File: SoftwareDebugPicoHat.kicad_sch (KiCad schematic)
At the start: 13 parts, among them J1 35362-0950, J2 Conn_Coaxial, J3 USB_C_Receptacle_USB2.0_14P, J4 Conn_Coaxial, J5 Conn_01x04_Pin, U1 RFM98PW, U3 LORA1280F27-TCXO

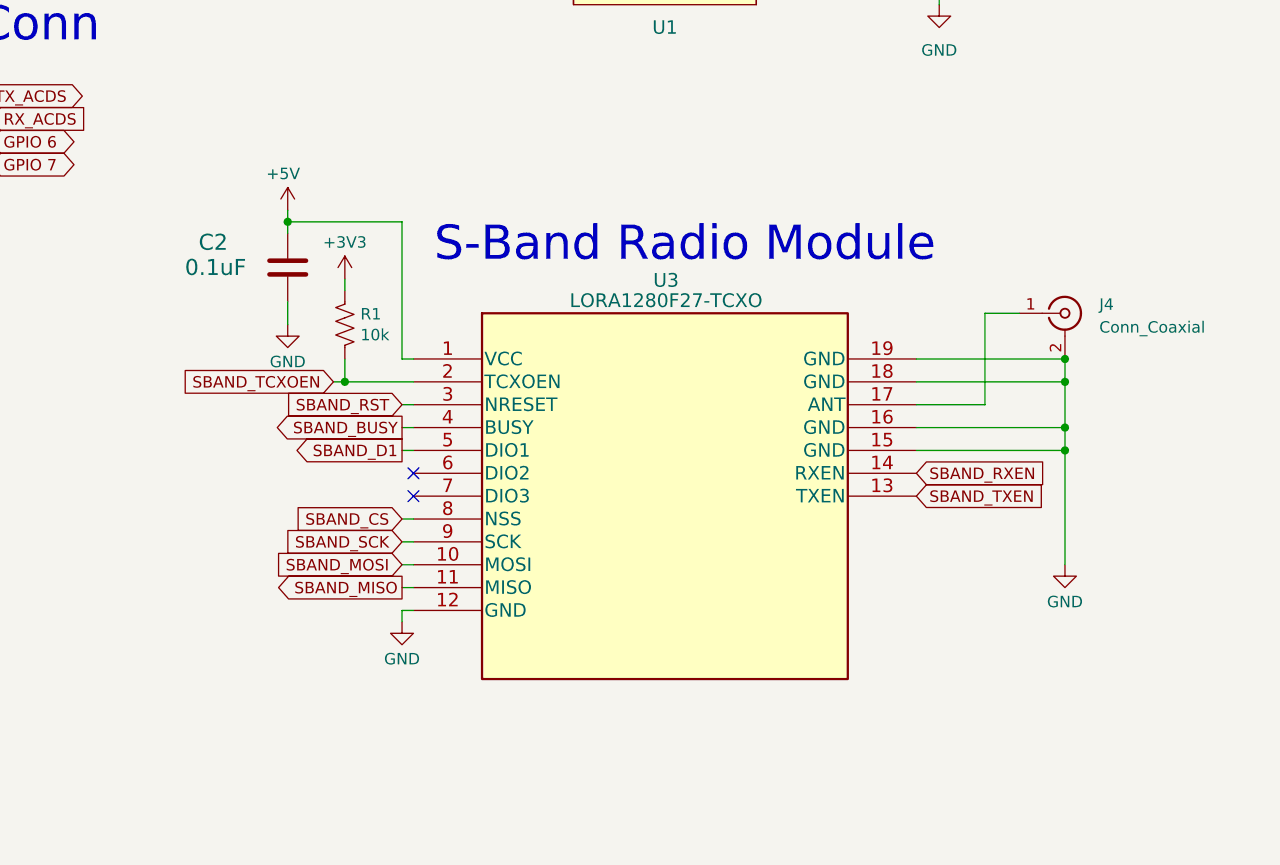
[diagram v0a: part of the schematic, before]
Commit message: Solving Samwise
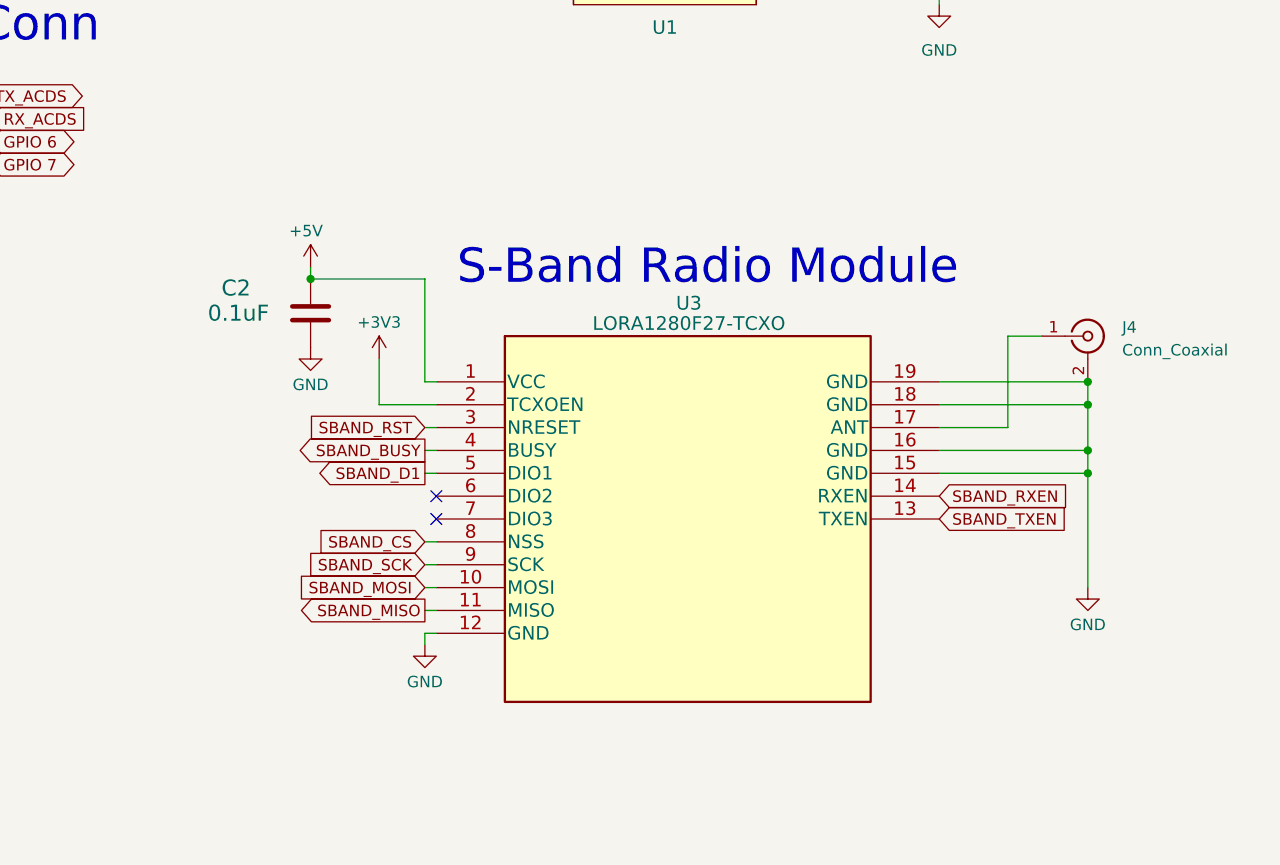
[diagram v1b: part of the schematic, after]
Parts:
- removed R1: 10k, Resistor_SMD:R_0603_1608Metric, symbol Device:R_US
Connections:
- net SBAND_TCXOEN is gone; now on net +3V3: U3.2 (TCXOEN)
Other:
- moved on the sheet: C2, J4, U3
